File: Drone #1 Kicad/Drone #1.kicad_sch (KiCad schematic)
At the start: 8 parts, among them SW1 SW_Nidec_CAS-120A1, U1 Pico, U2 NRF24L01_Breakout, U3 NRF24L01_Breakout

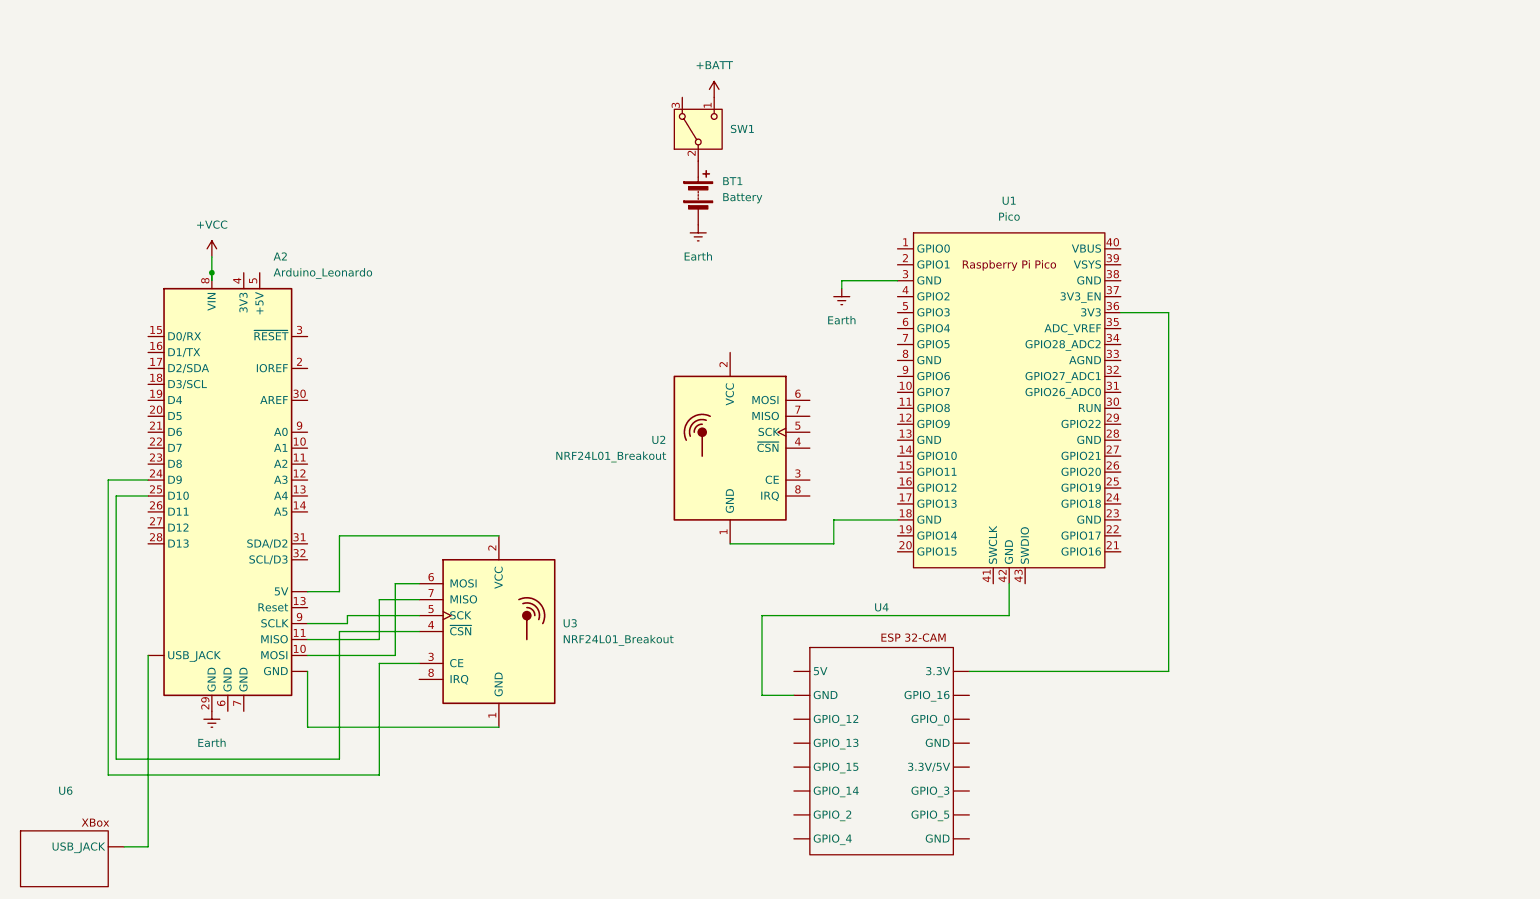
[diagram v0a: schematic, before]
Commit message: 5.20
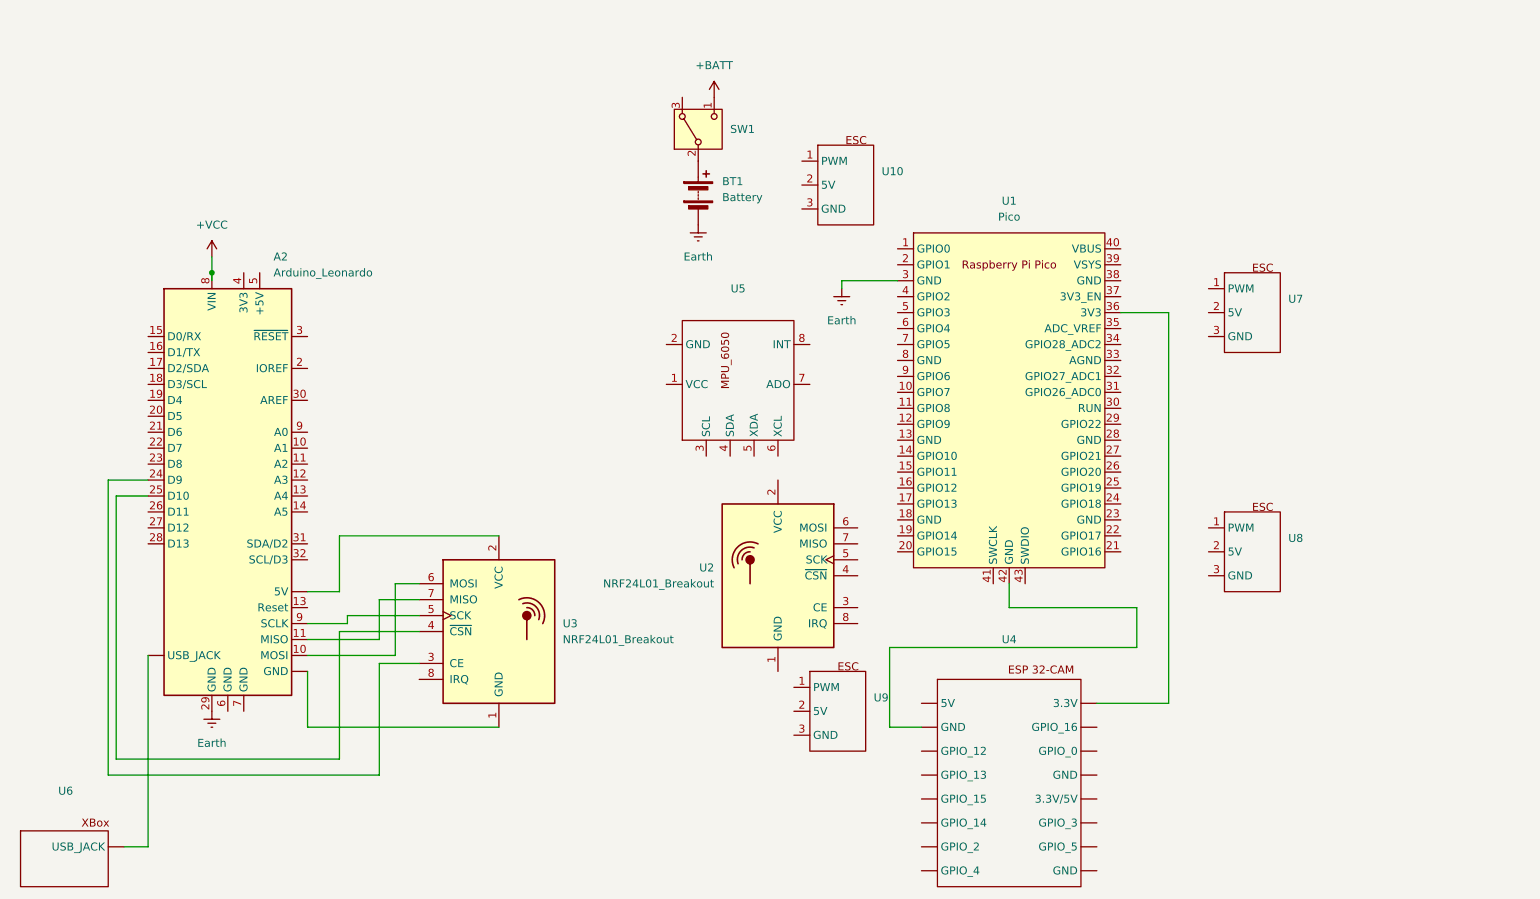
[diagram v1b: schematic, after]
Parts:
- added U10, U7, U8, U9: ~, symbol pcb_library:ESC
- added U5: ~, symbol pcb_library:MPU6050
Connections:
- net at U4. (GND): now also U1.42 (GND)
- net at U2.1 (GND): no longer U1.18 (GND)
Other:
- moved on the sheet: U2, U4

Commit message: 5.22
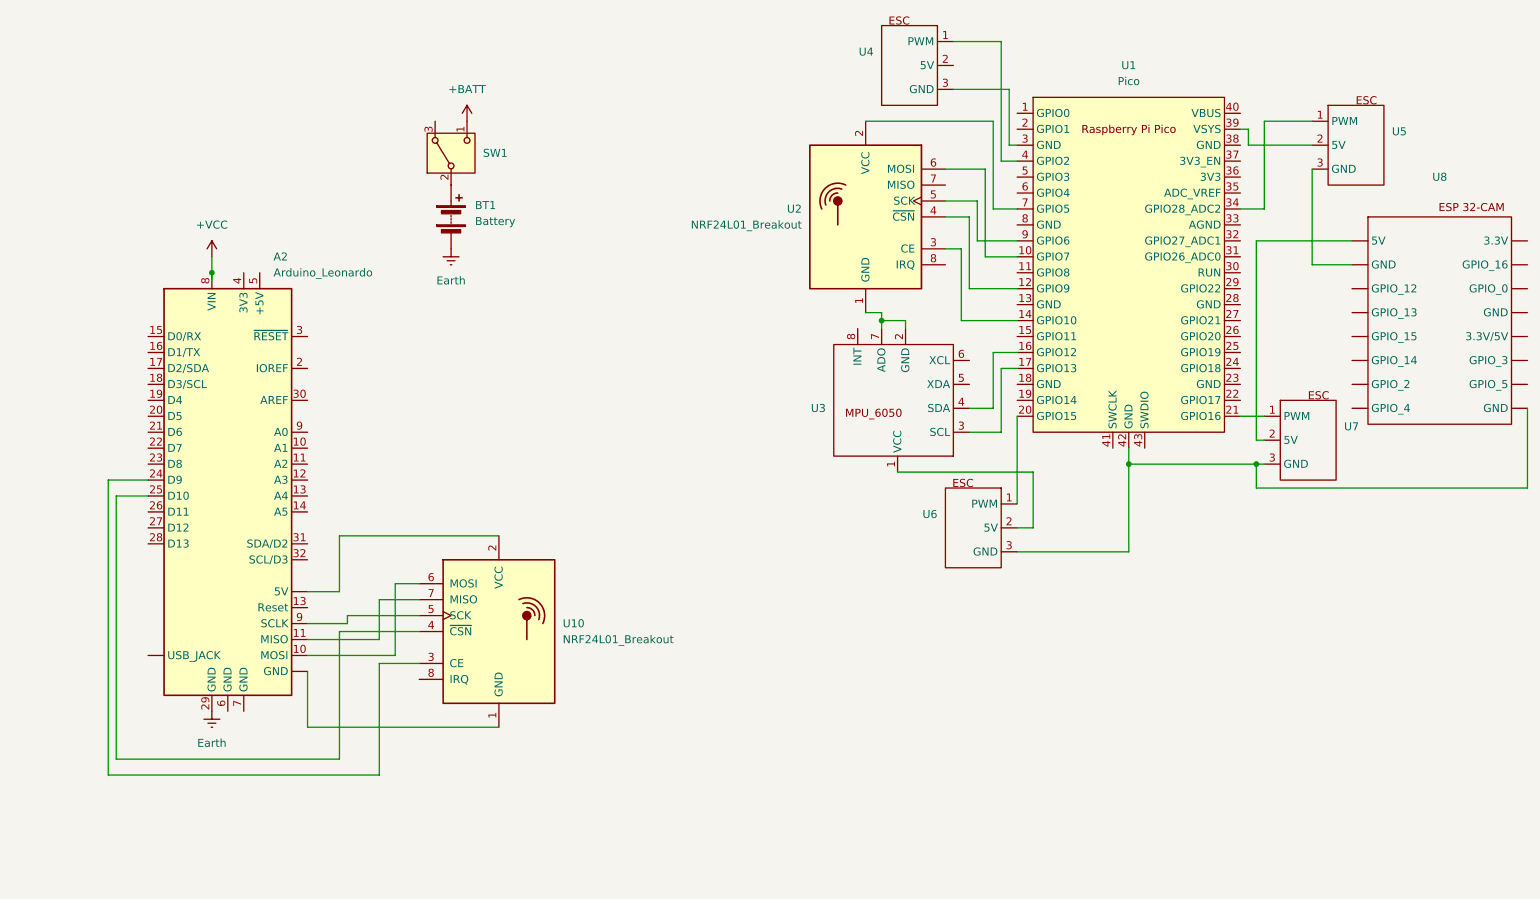
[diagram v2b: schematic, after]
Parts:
- removed U6: ~, symbol Drone Library:XBox
- renumbered U3 to U10, U5 to U3, U10 to U4, U7 to U5, U9 to U6, U8 to U7, U4 to U8
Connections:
- net Earth: no longer U1.3 (GND)
- net at U7.1 (PWM): now also U1.21 (GPIO16)
- net at U7.2 (5V): now also U8. (GND)
- net at U7.3 (GND): now also U1.42 (GND), U6.3 (GND), U8. (GND)
- net at U3.1 (VCC): now also U6.2 (5V)
- net at U3.2 (GND): now also U2.1 (GND), U3.7 (ADO)
- net at U3.3 (SCL): now also U1.17 (GPIO13)
- net at U3.4 (SDA): now also U1.16 (GPIO12)
- net at U4.1 (PWM): now also U1.4 (GPIO2)
- net at U4.3 (GND): now also U1.3 (GND)
- net at U5.1 (PWM): now also U1.34 (GPIO28_ADC2)
- net at U5.2 (5V): now also U1.39 (VSYS)
- net at U5.3 (GND): now also U8. (GND)
- net at U1.36 (3V3): no longer U8. (GND)
- net at U2.2 (VCC): now also U1.7 (GPIO5)
- net at U2.3 (CE): now also U1.14 (GPIO10)
- net at U2.4 (~{CSN}): now also U1.12 (GPIO9)
- net at U2.5 (SCK): now also U1.9 (GPIO6)
- net at U2.6 (MOSI): now also U1.10 (GPIO7)
- net at U6.1 (PWM): now also U1.20 (GPIO15)
- now unconnected: U8. (GND)
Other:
- moved on the sheet: BT1, SW1, U1, U2, U3, U4, U5, U6, U7, U8

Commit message: 5.23
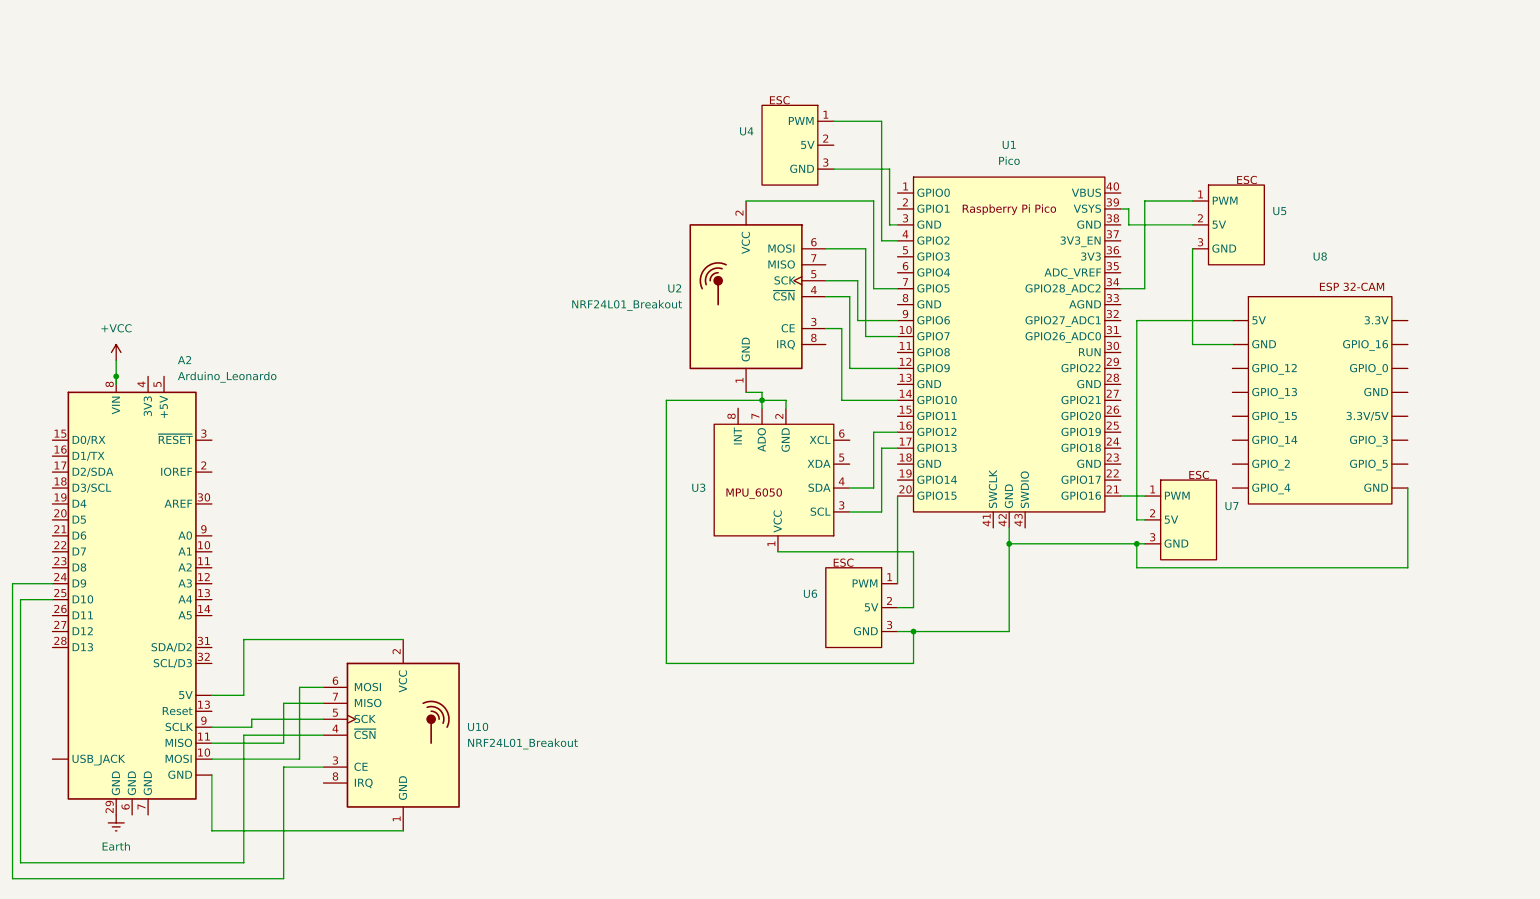
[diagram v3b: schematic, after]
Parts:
- removed BT1: Battery, symbol Device:Battery
- removed SW1: SW_Nidec_CAS-120A1, Button_Switch_SMD:Nidec_Copal_CAS-120A, symbol Switch:SW_Nidec_CAS-120A1
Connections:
- net at U1.42 (GND), U6.3 (GND), U7.3 (GND)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: now also U2.1 (GND), U3.2 (GND), U3.7 (ADO)
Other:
- title: (none) -> IFLY V2
- moved on the sheet: A2, U1, U10, U2
